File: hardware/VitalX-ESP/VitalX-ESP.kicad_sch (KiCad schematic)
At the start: 56 parts, among them J1 ECG Probe, J2 GSR Probe, J3 UART, J4 JTAG, J5 Power terminal, Q1 BSS138, SW2 Reset, U1 AD8232ACPZ-R7, U3 ADP160AUJZ-1.8-R7, U4 ADPD144RI-ACEZ-RL, U5 AMS1117-3.3, U6 MCP601-xOT, U7 ESP32-S2-WROOM

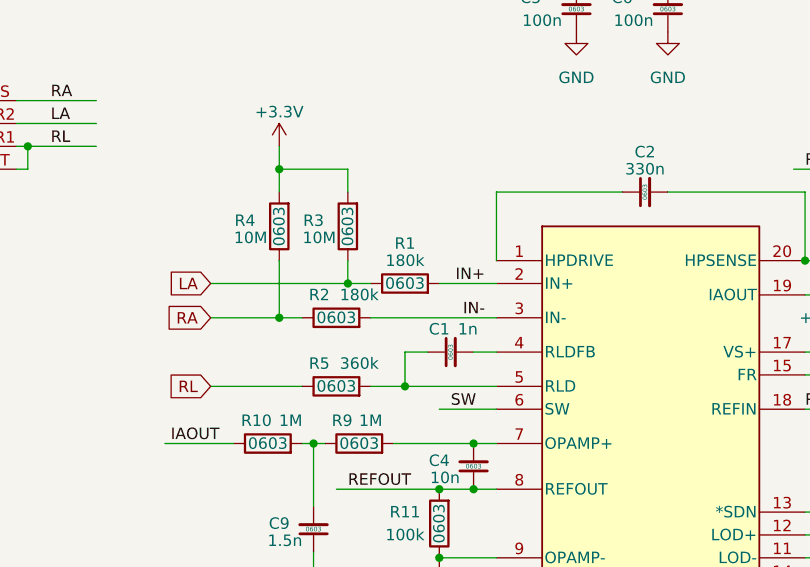
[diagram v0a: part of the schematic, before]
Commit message: [nightly] Initial PCB layout.
4 layer stack up:
- Signal
- GND
- GND
- Signal
Currently working on ECG Block.
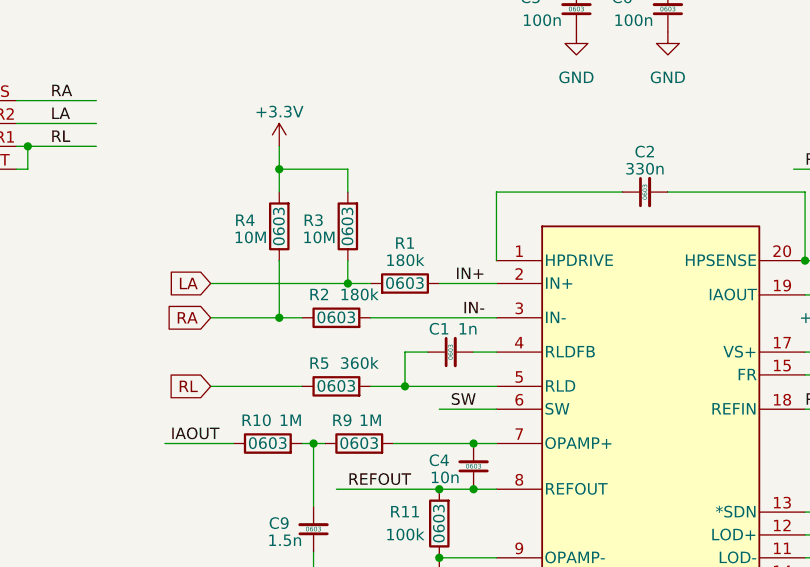
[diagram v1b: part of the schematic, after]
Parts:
- J1: footprint Connector_Audio:Jack_3.5mm_PJ320D_Horizontal -> AUDIO_SJ2-3593D-SMT-TR:SJ2-3593D-SMT-TR
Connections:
- net IN+: now also R1.1; no longer R1.2
- net LA: now also R1.2; no longer R1.1
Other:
- moved on the sheet: R1
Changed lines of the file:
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@@
       (effects (font (size 1.27 1.27)))
     )
-    (property "Footprint" "Connector_Audio:Jack_3.5mm_PJ320D_Horizontal" (at 40.005 198.755 0)
+    (property "Footprint" "AUDIO_SJ2-3593D-SMT-TR:SJ2-3593D-SMT-TR" (at 40.005 198.755 0)
       (effects (font (size 1.27 1.27)) hide)
     )
@@
     )
   )
-  (symbol (lib_id "Device:R") (at 88.265 216.535 90) (unit 1)
+  (symbol (lib_id "Device:R") (at 88.265 216.535 270) (mirror x) (unit 1)
     (in_bom yes) (on_board yes) (dnp no)
     (property "Reference" "R1" (at 88.265 212.09 90)
